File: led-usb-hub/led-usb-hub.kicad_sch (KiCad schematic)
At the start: 27 parts, among them J1 USB_C_Receptacle_USB2.0, J2 USB_A_RGB, J3 USB_A_RGB, J4 USB_A_RGB, SW1 SW_Push, U1 SL2.1A, U2 KB2040, Y1 12MHz

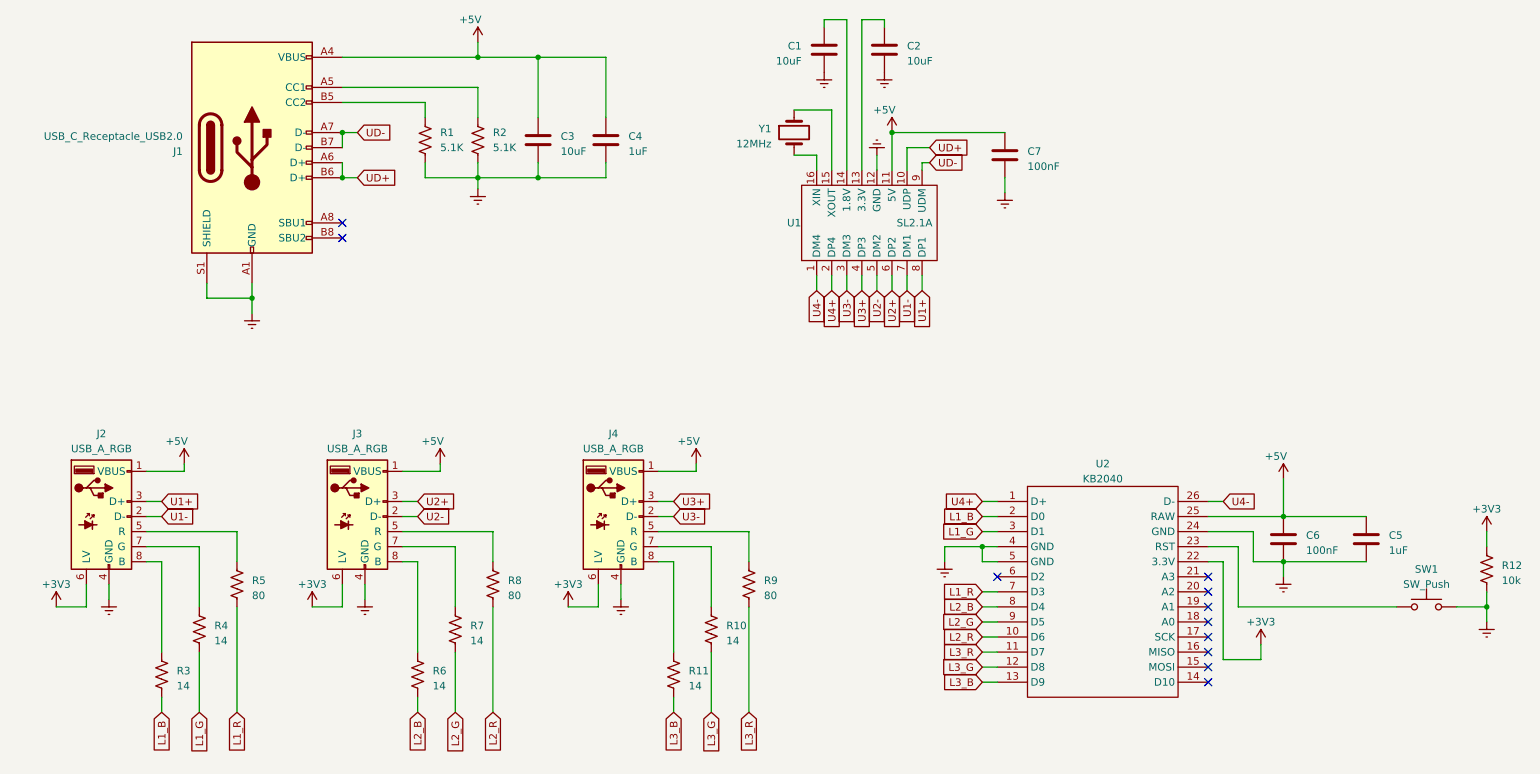
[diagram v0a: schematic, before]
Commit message: finish routing NEED: graphics and labels
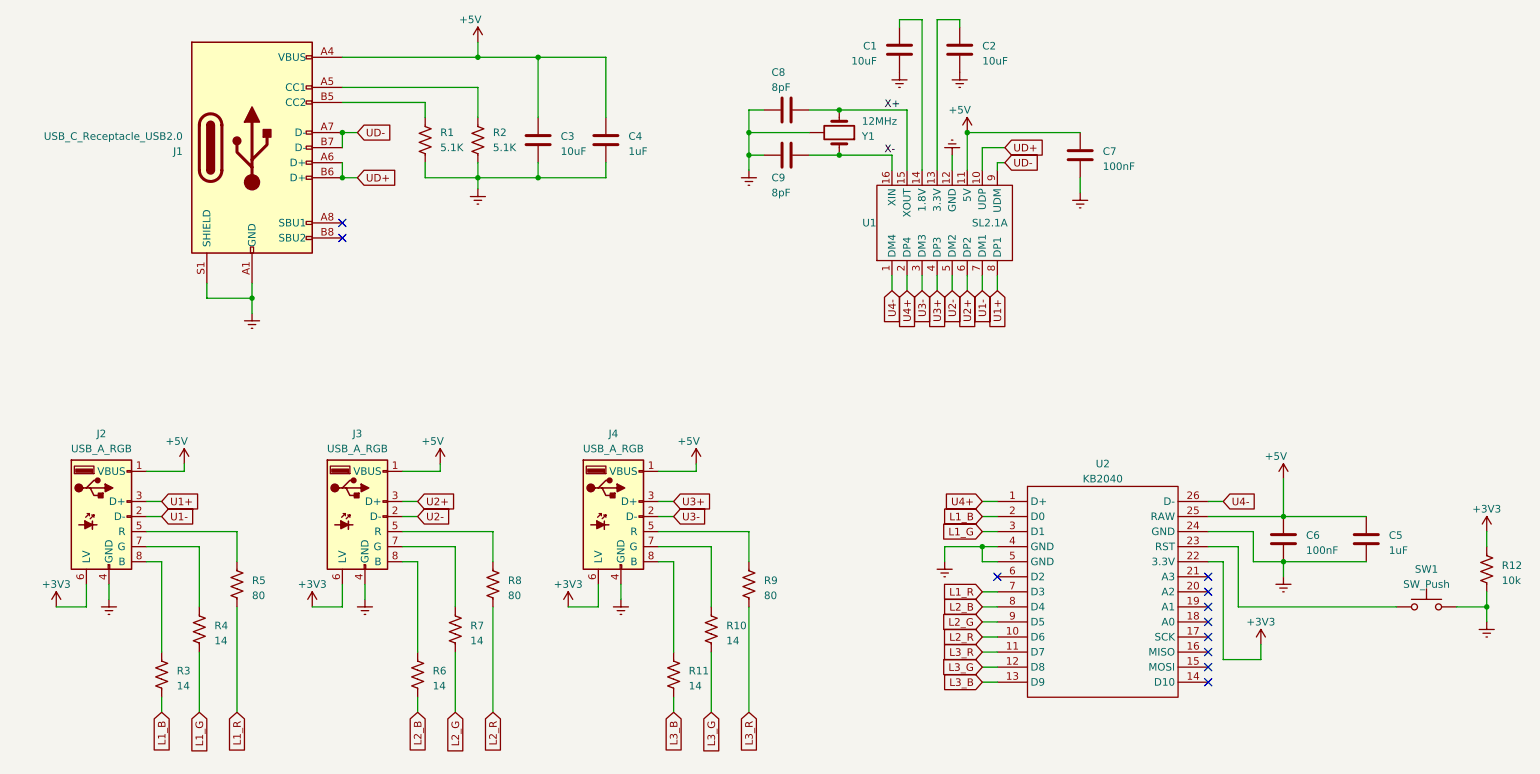
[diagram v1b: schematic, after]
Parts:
- added C8, C9: 8pF, Capacitor_SMD:C_0603_1608Metric_Pad1.08x0.95mm_HandSolder, symbol Device:C
- SW1: footprint (none) -> kss_switch:SW_KSS241GLFS_CNK
- Y1: footprint (none) -> ecs_osc:XTAL_ECS-120-8-33-JGN-TR3
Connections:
- net Earth: now also SW1.1, Y1.2 (GND), Y1.4 (GND), C8.2, C9.2; no longer SW1.2
- net at U2.23 (RST): now also SW1.2; no longer SW1.1
- net X+: now reaches U1.15 (XOUT)
- net X+: now also Y1.3, C8.1; no longer Y1.1
- net X-: now reaches U1.16 (XIN)
- net X-: now also Y1.1, C9.1; no longer Y1.2
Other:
- moved on the sheet: C1, C2, C7, U1
